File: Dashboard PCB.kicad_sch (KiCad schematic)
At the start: 20 parts, among them J1 Controls_Leader_Export_02x06, J2 Conn_01x02, J3 Conn_01x02, J4 FAN_CTRL_01x02

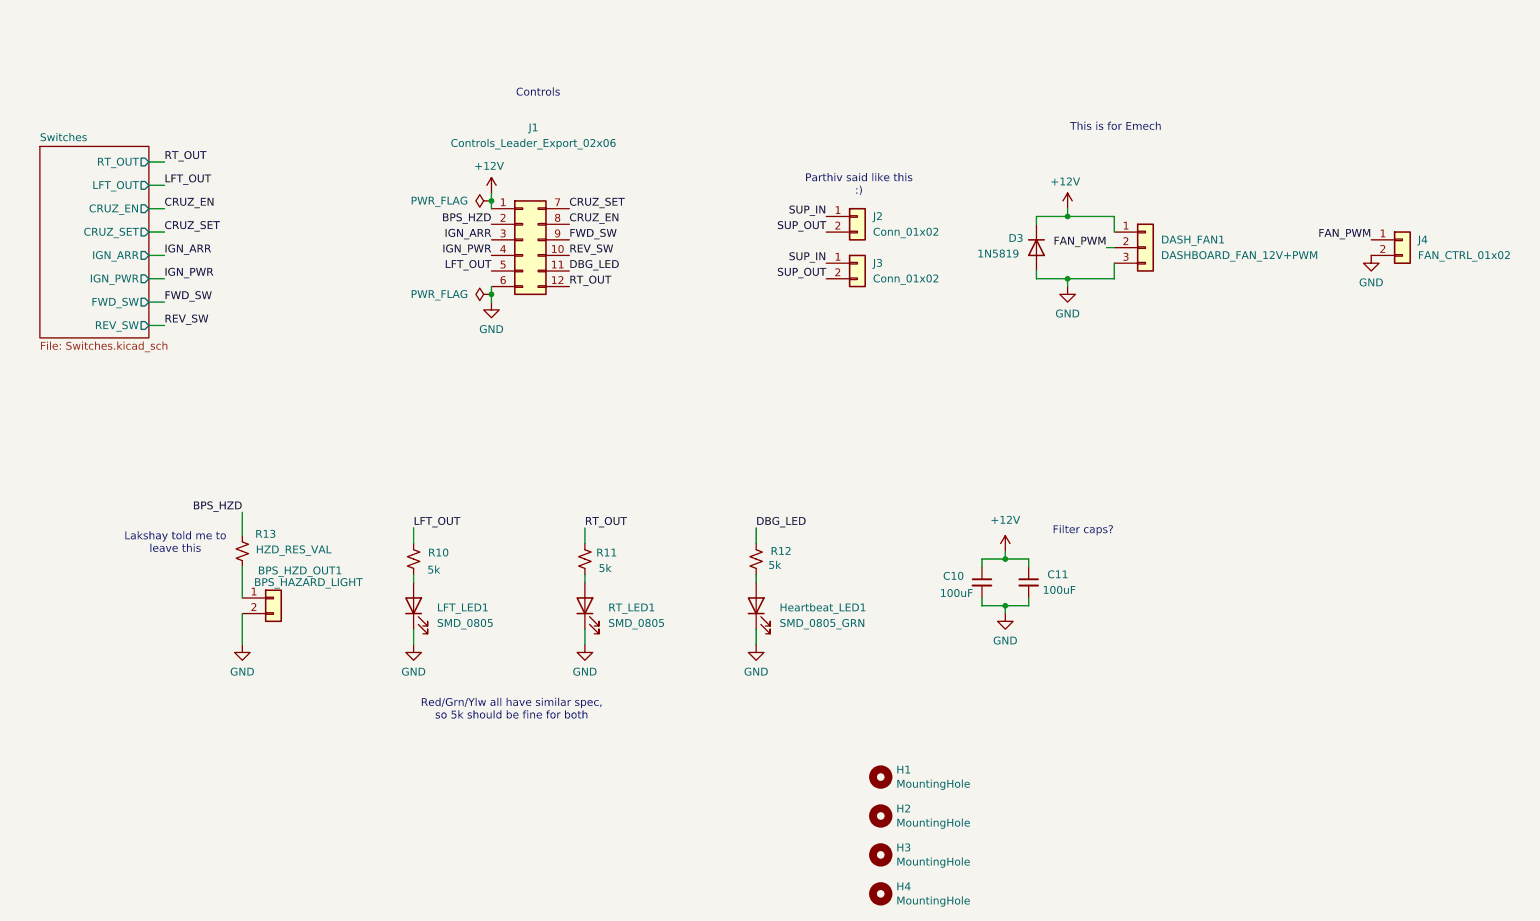
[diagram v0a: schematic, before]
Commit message: Made pretty
Fixed a few things up and made it pretty.
Still need to double check a few things and assign all footprints
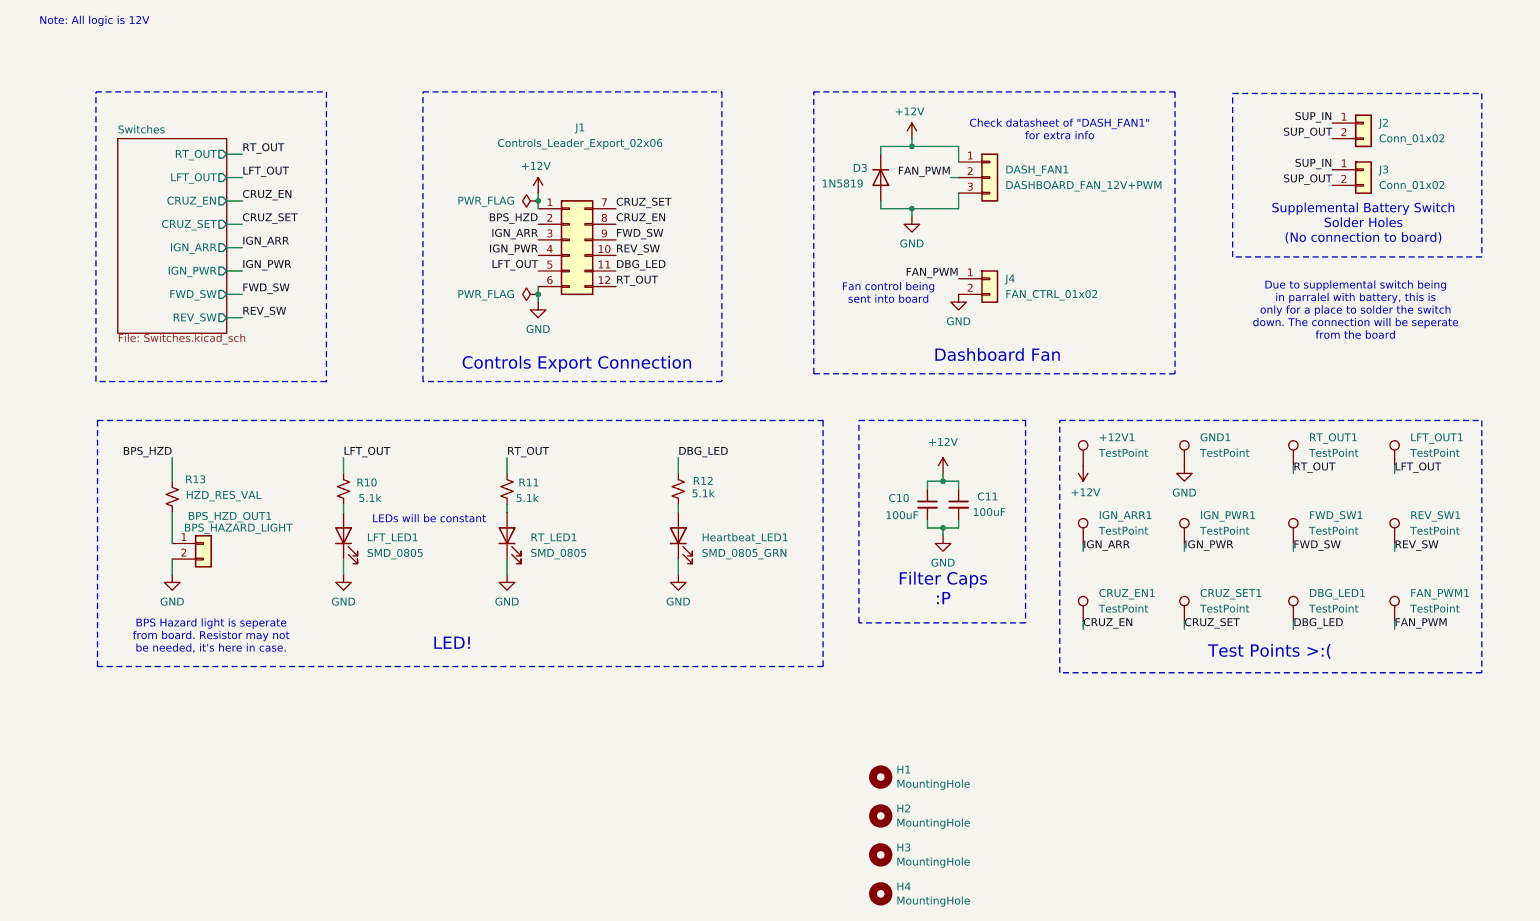
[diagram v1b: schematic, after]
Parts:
- added +12V1, CRUZ_EN1, CRUZ_SET1, DBG_LED1, FAN_PWM1, FWD_SW1, GND1, IGN_ARR1, IGN_PWR1, LFT_OUT1, REV_SW1, RT_OUT1: TestPoint, symbol Connector:TestPoint
- R10, R11, R12: value 5k -> 5.1k
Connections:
- net +12V: now also +12V1.1
- net CRUZ_EN: now also CRUZ_EN1.1
- net CRUZ_SET: now also CRUZ_SET1.1
- net DBG_LED: now also DBG_LED1.1
- net FAN_PWM: now also FAN_PWM1.1
- net FWD_SW: now also FWD_SW1.1
- net GND: now also GND1.1
- net IGN_ARR: now also IGN_ARR1.1
- net IGN_PWR: now also IGN_PWR1.1
- net LFT_OUT: now also LFT_OUT1.1
- net REV_SW: now also REV_SW1.1
- net RT_OUT: now also RT_OUT1.1
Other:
- note added: "BPS Hazard light is seperate from board. Resistor may not be needed, it's here in case."
- note added: "Check datasheet of "DASH_FAN1" for extra info"
- note added: "Controls Export Connection"
- note added: "Dashboard Fan"
- note added: "Due to supplemental switch being in parralel with battery, this is only for a place to solder the switch down. The connection will be seperate from the board"
- note added: "Fan control being sent into board"
- note added: "Filter Caps :P"
- note added: "LED!"
- note added: "LEDs will be constant"
- note added: "Note: All logic is 12V"
- note added: "Supplemental Battery Switch Solder Holes (No connection to board)"
- note added: "Test Points >:("
- note removed: "Controls"
- note removed: "Filter caps?"
- note removed: "Lakshay told me to leave this"
- note removed: "Parthiv said like this :)"
- note removed: "Red/Grn/Ylw all have similar spec, so 5k should be fine for both"
- note removed: "This is for Emech"
- moved on the sheet: BPS_HZD_OUT1, C10, C11, D3, DASH_FAN1, Heartbeat_LED1, J1, J2, J3, J4, LFT_LED1, R10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
